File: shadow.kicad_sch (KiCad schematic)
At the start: 12 parts, among them SW1 SW_Push, SW2 SW_Push

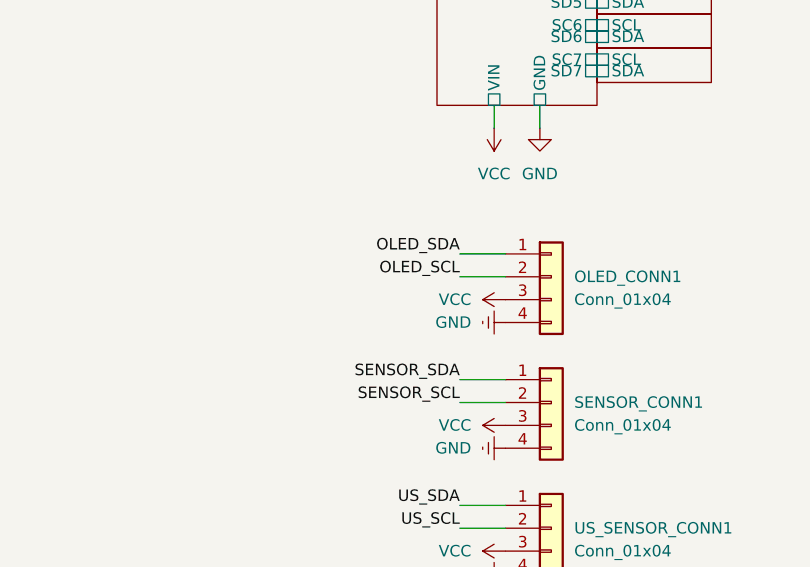
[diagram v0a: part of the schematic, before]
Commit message: start work on pcb design
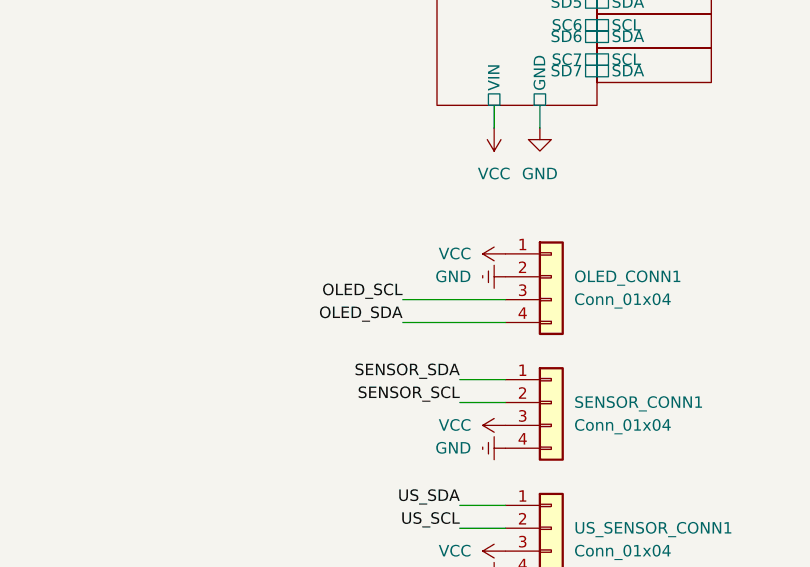
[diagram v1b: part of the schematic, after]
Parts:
- GPIO_L1, GPIO_R1, PICO_L1, PICO_R1: footprint Connector_PinSocket_1.00mm:PinSocket_1x15_P1.00mm_Vertical -> Connector_PinSocket_2.54mm:PinSocket_1x15_P2.54mm_Vertical
- MOTOR_CONN1: footprint Connector_PinSocket_1.00mm:PinSocket_1x02_P1.00mm_Vertical -> Connector_PinSocket_2.54mm:PinSocket_1x02_P2.54mm_Vertical
- OLED_CONN1, SENSOR_CONN1: footprint Connector_PinSocket_1.00mm:PinSocket_1x04_P1.00mm_Vertical -> Connector_PinSocket_2.54mm:PinSocket_1x04_P2.54mm_Vertical
- RST_SW1, SW1, SW2: footprint Button_Switch_THT:SW_PUSH-12mm -> Button_Switch_THT:SW_PUSH_6mm
- UART1: footprint Connector_PinHeader_1.00mm:PinHeader_1x03_P1.00mm_Vertical -> Connector_PinSocket_2.54mm:PinSocket_1x03_P2.54mm_Vertical
- US_SENSOR_CONN1: footprint Connector_PinHeader_1.00mm:PinHeader_1x04_P1.00mm_Vertical -> Connector_PinSocket_2.54mm:PinSocket_1x04_P2.54mm_Vertical
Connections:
- net GND: now also OLED_CONN1.2 (Pin_2); no longer OLED_CONN1.4 (Pin_4)
- net OLED_SCL: now also OLED_CONN1.3 (Pin_3); no longer OLED_CONN1.2 (Pin_2)
- net OLED_SDA: now also OLED_CONN1.4 (Pin_4); no longer OLED_CONN1.1 (Pin_1)
- net VCC: now also OLED_CONN1.1 (Pin_1); no longer OLED_CONN1.3 (Pin_3)
